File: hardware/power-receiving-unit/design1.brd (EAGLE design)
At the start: 55 x 40 mm, 81 parts, among them IC12 NRF52832, IC3 TPS54308DDCR, IC4 MCP6486T-E/OT, Q1 BSS138, Q2 SI3481DV, Y1 32MHz, Y2 32.768kHz

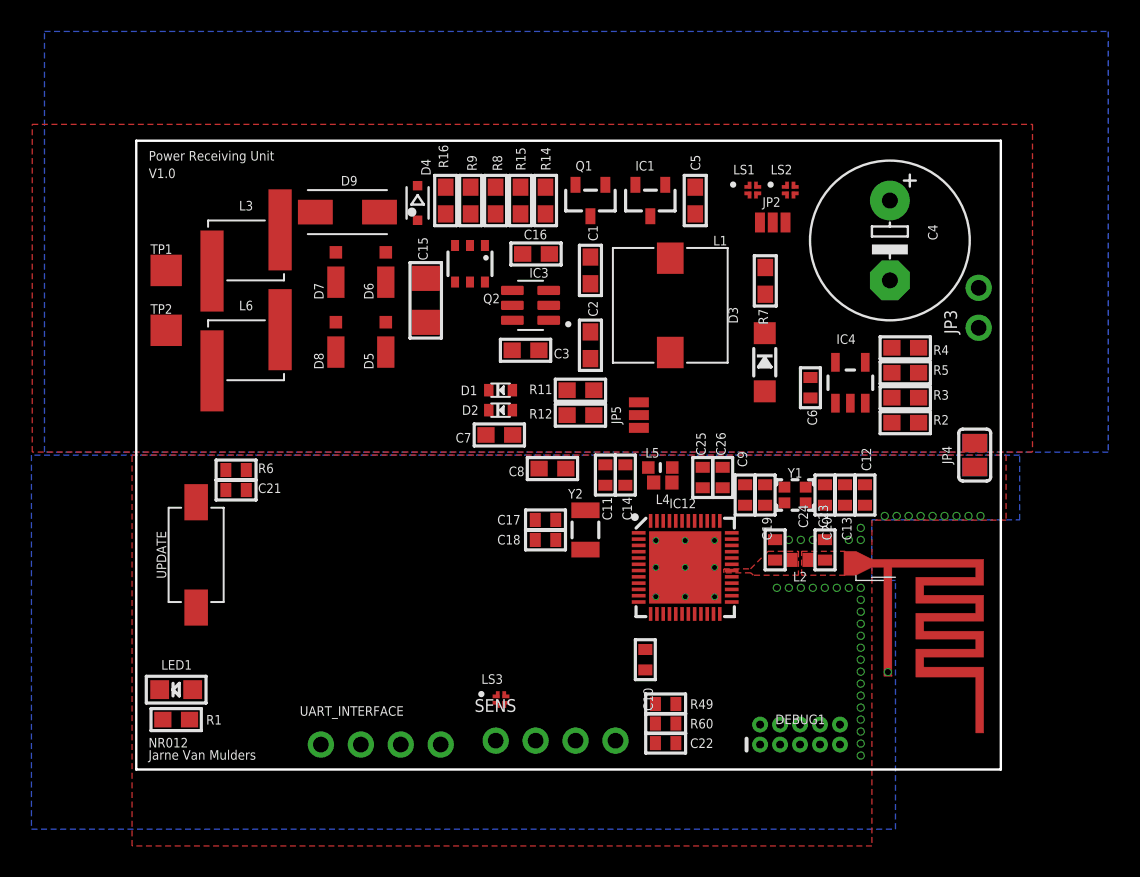
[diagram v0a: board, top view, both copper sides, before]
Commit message: power receiving unit PCB V1.0 ready
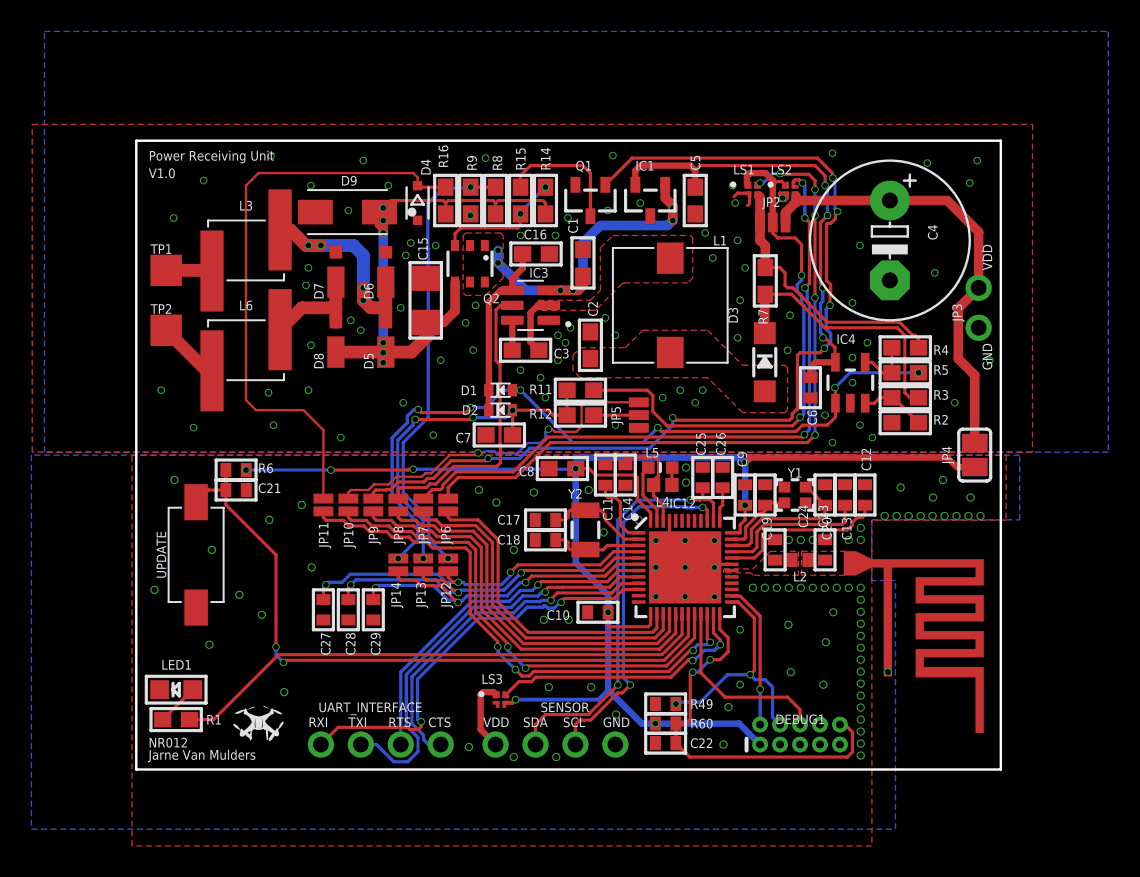
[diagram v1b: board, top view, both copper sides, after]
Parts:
- removed SENS: (no value), microbuilder:1X04_ROUND
- added C27, C28, C29: 100n, microbuilder:0402
- added JP10, JP11, JP12, JP13, JP14, JP6, JP7, JP8, JP9: JUMPER-SMT_2_NO_NO-SILK, SparkFun-Jumpers:SMT-JUMPER_2_NO_NO-SILK
- added SENSOR: (no value), microbuilder:1X04_ROUND
- moved C10 4.27 mm to (29.4, 10.0), turned to 180 degrees
- moved C1 0.67 mm to (28.4, 32.2), turned to 90 degrees
- moved C8 0.64 mm to (27.1, 19.1)
- moved L4 0.16 mm to (33.5, 18.1)
- turned C14 to 90 degrees
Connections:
- new net P02: C27.1, IC12.4, JP12.1
- new net P03: C28.1, IC12.5, JP13.1
- new net P04: C29.1, IC12.6, JP14.1
- new net P11: IC12.14, JP6.1
- new net P12: IC12.15, JP7.1
- new net P13: IC12.16, JP8.1
- new net P14: IC12.17, JP9.1
- new net P17: IC12.20, JP10.1
- new net P19: IC12.22, JP11.1
- net ADC1: now also JP12.2; no longer IC12.4
- net BUCK_EN: now also JP8.2; no longer IC12.16
- net EN1: now also JP6.2; no longer IC12.14
- net EN2: now also JP7.2; no longer IC12.15
- net GND: now also C27.2, C28.2, C29.2, SENSOR.4; no longer SENS.4
- net I2C_SCL: now also SENSOR.3; no longer SENS.3
- net I2C_SDA: now also SENSOR.2; no longer SENS.2
- net PG: now also JP9.2; no longer IC12.17
- net PWM-CHG: now also JP10.2; no longer IC12.20
- net V-ICHG: now also JP14.2; no longer IC12.6
- net V-VCHG: now also JP13.2; no longer IC12.5
- net VDD_SENS: now also SENSOR.1; no longer SENS.1
- net WAKE-UP: now also JP11.2; no longer IC12.22
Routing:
- net VDD_BLE: track 0.00 -> 97.2 mm, vias 0 -> 9
- net PG: track 0.00 -> 63.2 mm, vias 0 -> 6
- net V-ICHG: track 0.00 -> 49.1 mm, vias 0 -> 7
- net EN1: track 0.00 -> 45.9 mm, vias 0 -> 6
- net P16: track 0.00 -> 43.9 mm, vias 0 -> 2
- net EN2: track 0.00 -> 43.7 mm, vias 0 -> 4
- net WAKE-UP: track 0.00 -> 37.4 mm
- net VDD_WPT: track 0.00 -> 35.9 mm, vias 0 -> 6
- net VMEAS: track 0.00 -> 35.6 mm, vias 0 -> 2
- net LED: track 0.00 -> 34.9 mm
- net P19: track 0.00 -> 34.7 mm, vias 0 -> 4
- net P17: track 0.00 -> 31.3 mm, vias 0 -> 2
- net 3.3V: track 0.00 -> 29.8 mm, vias 0 -> 4
- net ADC1: track 0.00 -> 29.2 mm, vias 0 -> 2
- net VCHG: track 0.00 -> 29.1 mm
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- added copper zone on layer 1, net N$13
- added copper zone on layer 1, net N$3
- added copper zone on layer 1, net VIN
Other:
- board text added: "CTS"
- board text added: "GND"
- board text added: "RTS"
- board text added: "RXI"
- board text added: "SCL"
- board text added: "SDA"
- board text added: "TXI"
- board text added: "VDD"
